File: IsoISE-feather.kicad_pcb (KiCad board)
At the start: 2 copper layers, 50.8 x 22.9 mm, 119 parts, among them J1 Conn_01x03, J2 BNC, J3 FEATHER, U1 MTU1D0305MC, U2 ADUM1250ARZ, U3 MCP4017, U4 TL072, U5 REF3130, U6 MCP3221

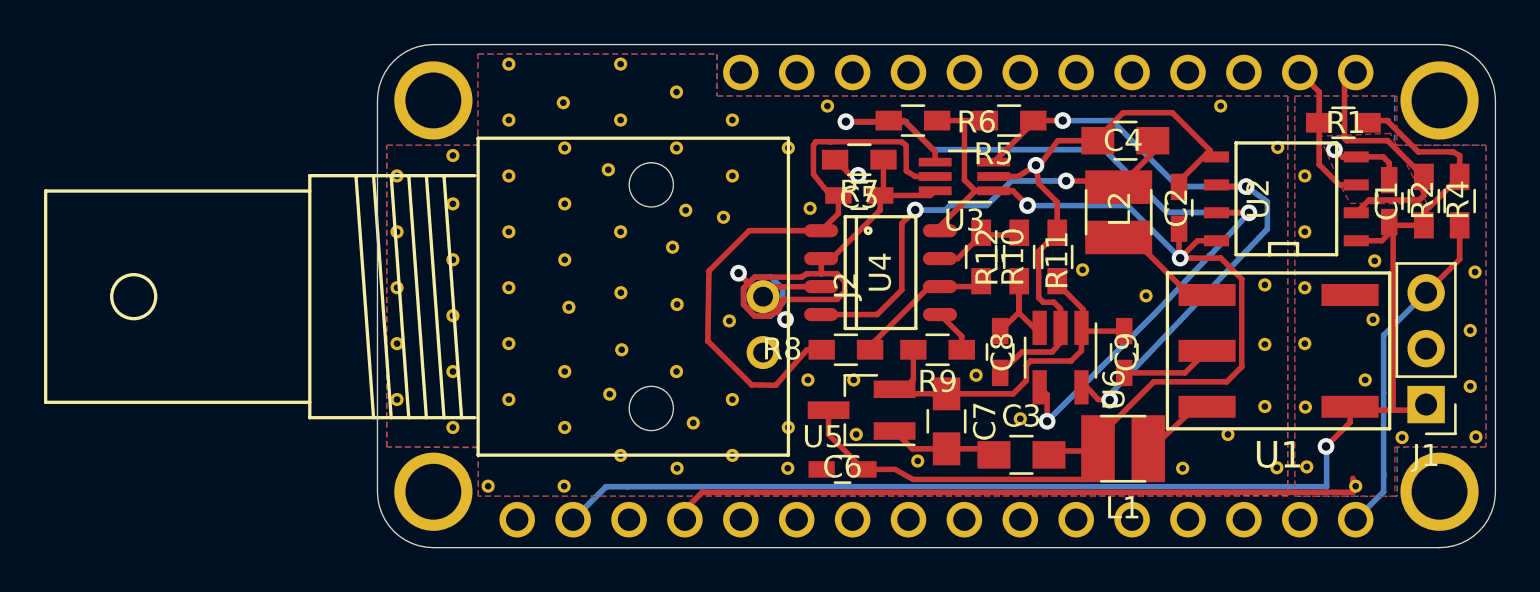
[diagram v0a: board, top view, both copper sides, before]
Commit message: files as submitted to oshpark
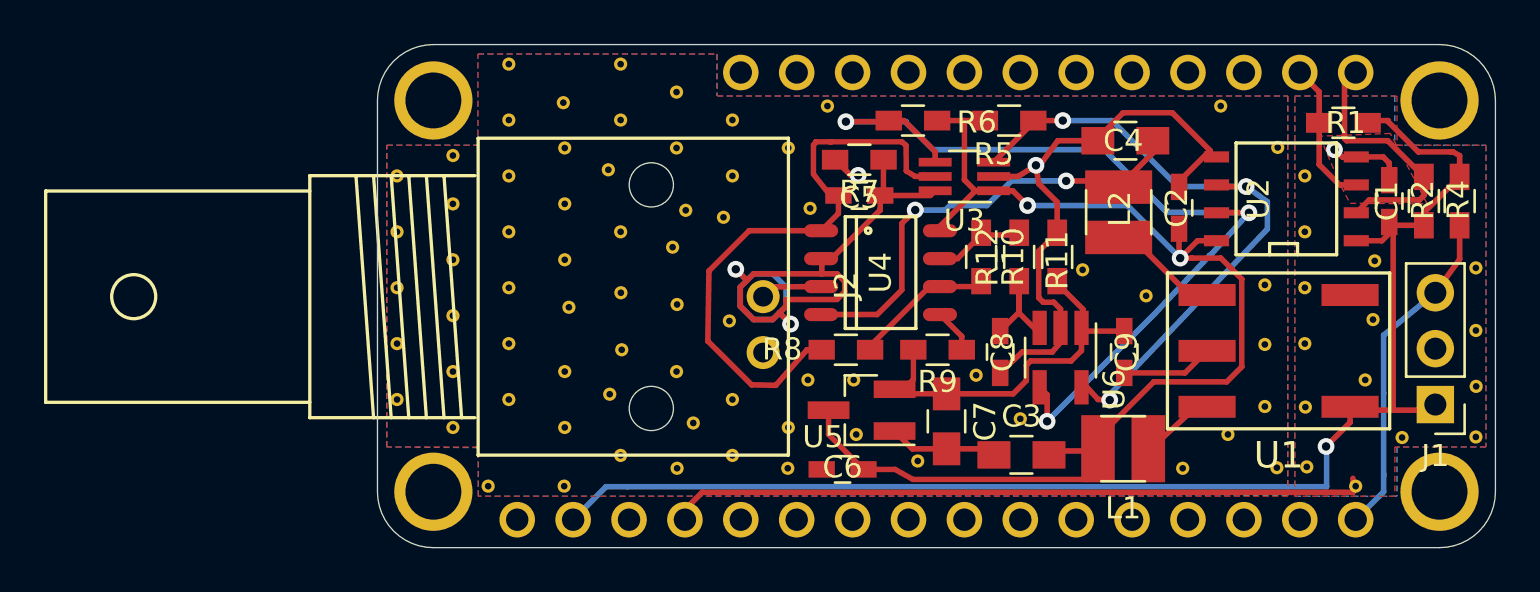
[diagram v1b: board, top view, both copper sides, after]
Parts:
- moved J1 0.42 mm to (170.6, 110.4)
- moved REF** 0.27 mm to (172.5, 109.6)
- moved REF** 0.25 mm to (172.4, 107.0)
- moved REF** 0.19 mm to (172.4, 104.2)
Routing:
- net Net-(C5-Pad2): track 29.1 -> 30.5 mm
